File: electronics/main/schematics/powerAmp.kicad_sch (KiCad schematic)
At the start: 15 parts, among them U27 CR1/2W-220K±5%-XT52, U28 CR1/2W-220K±5%-XT52, U29 CR-L5W-1KΩJ, U30 CR-L5W-1KΩJ

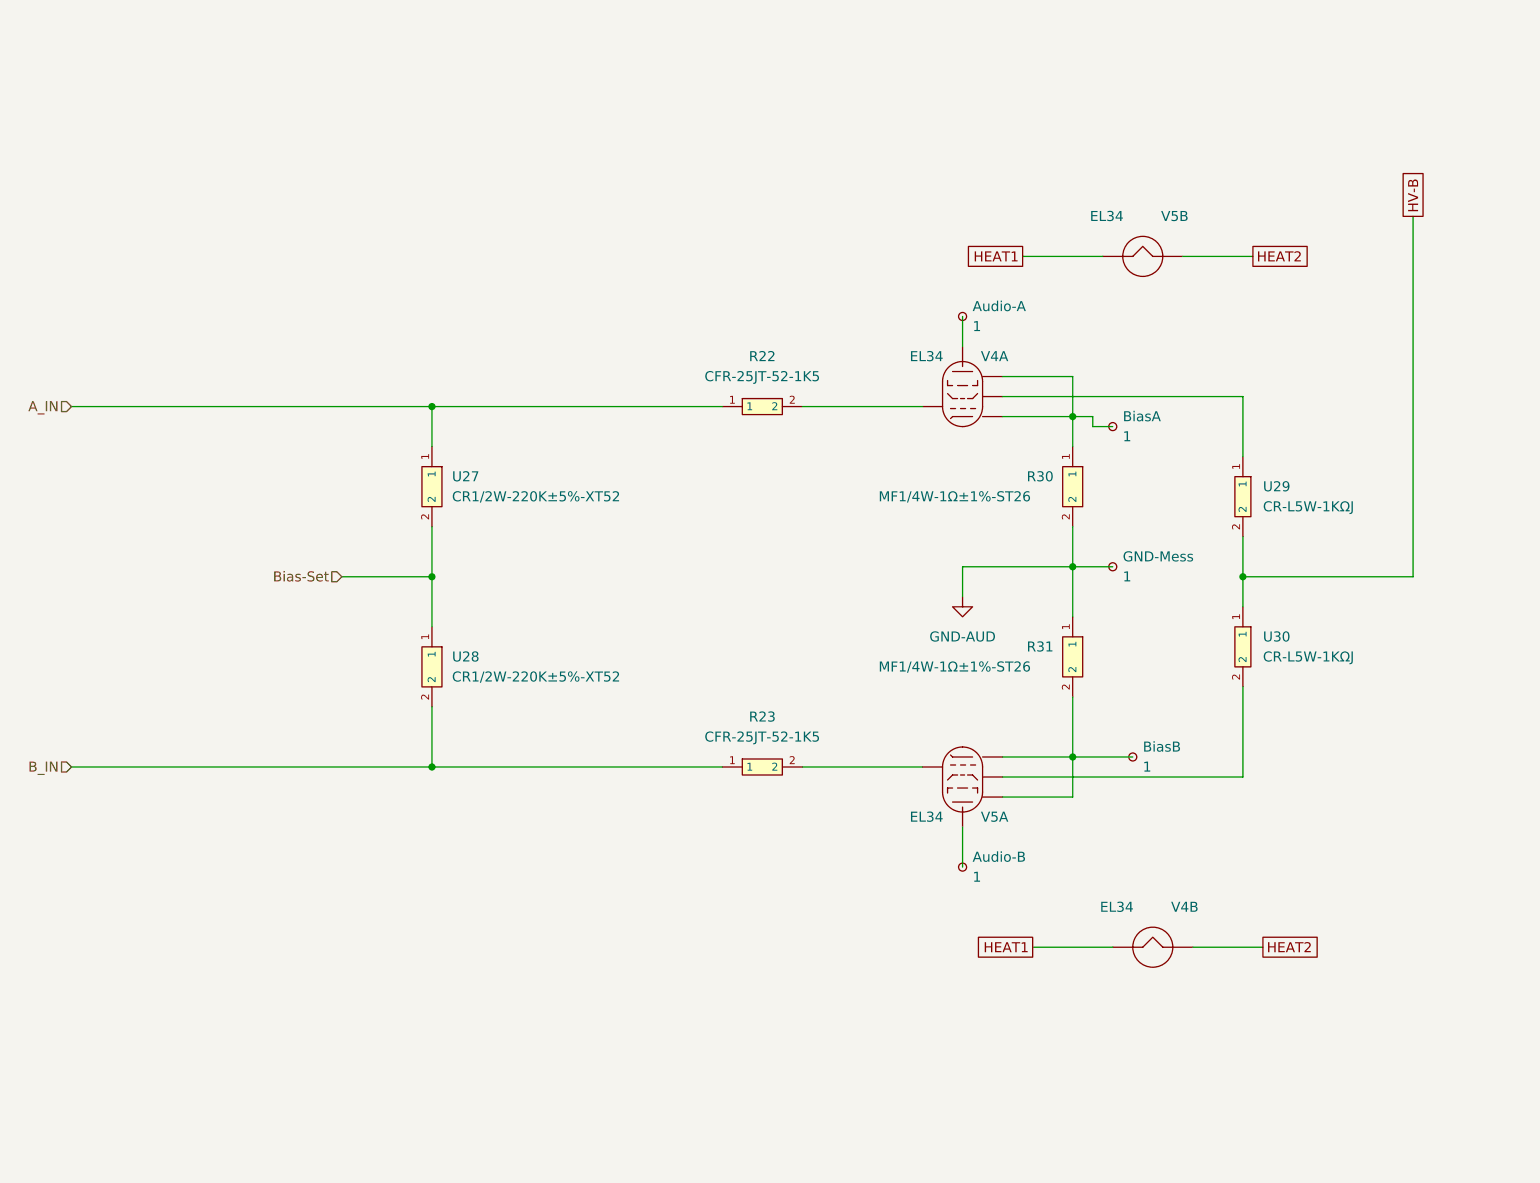
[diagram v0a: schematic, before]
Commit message: schematic  checked!
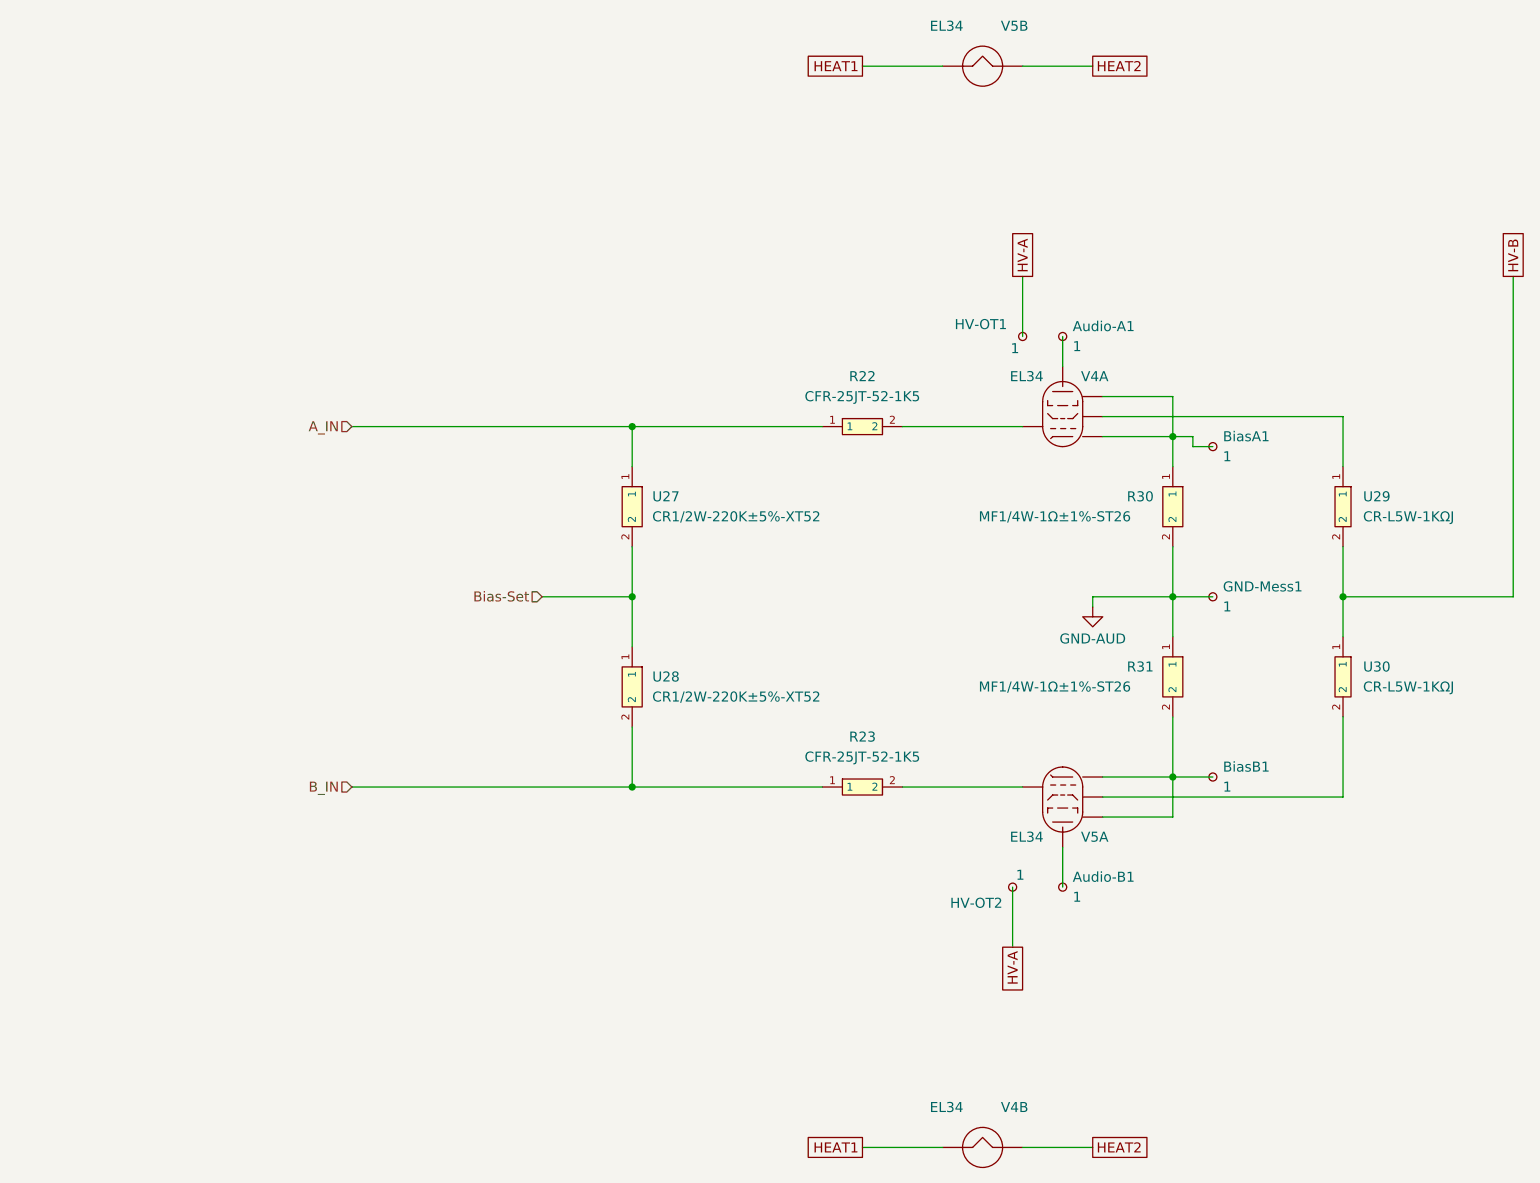
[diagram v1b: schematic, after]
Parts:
- added HV-OT1, HV-OT2: 1, TestPoint:TestPoint_THTPad_D3.0mm_Drill1.5mm, symbol Connector:TestPoint_Small
- renumbered Audio-A to Audio-A1, Audio-B to Audio-B1, BiasA to BiasA1, BiasB to BiasB1, GND-Mess to GND-Mess1
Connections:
- new net HV-A: HV-OT1.1, HV-OT2.1
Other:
- moved on the sheet: Audio-A1, Audio-B1, BiasA1, BiasB1, GND-Mess1, R22, R23, R30, R31, U27, U28, U29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
